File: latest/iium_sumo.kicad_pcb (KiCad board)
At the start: 2 copper layers, 56 parts, among them J1 I2C_VL53_1, J10 Cytron MD, J11 Cytron Start Module, J12 Conn_01x04, J13 Conn_01x04, J14 Conn_01x04, J15 EXTRA1, J16 Conn_01x02_Pin, J17 Conn_01x02_Pin, J18 UART1, J19 UART2, J2 I2C_VL53_2, J3 I2C_VL53_3, J4 I2C_VL53_4, J5 I2C_VL53_5, J6 IR_1, J7 IR_2, J8 IR_3, J9 IR_4, SW1 SW_SPST, SW2 SW_SPST, U1 TPS54360DDA, U4 Black Pill v2, U5 LM3940

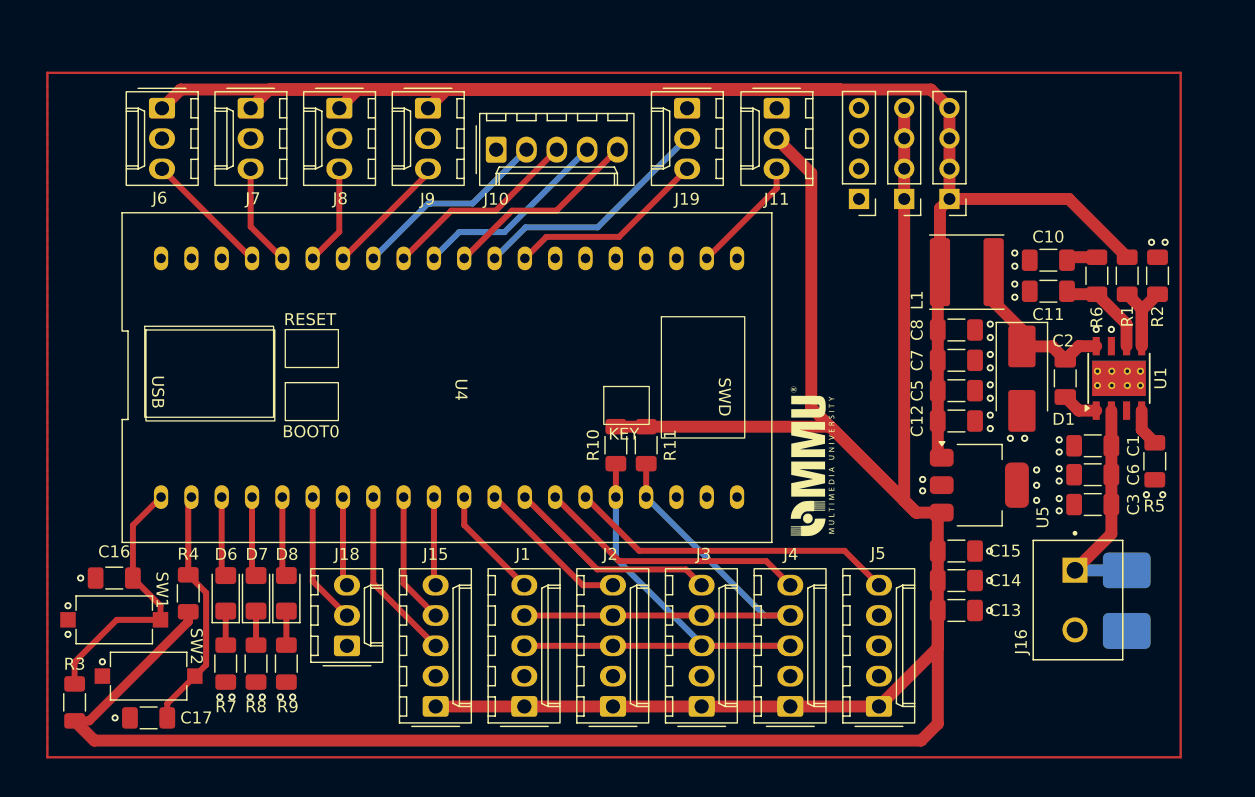
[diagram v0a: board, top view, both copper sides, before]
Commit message: drc cleared
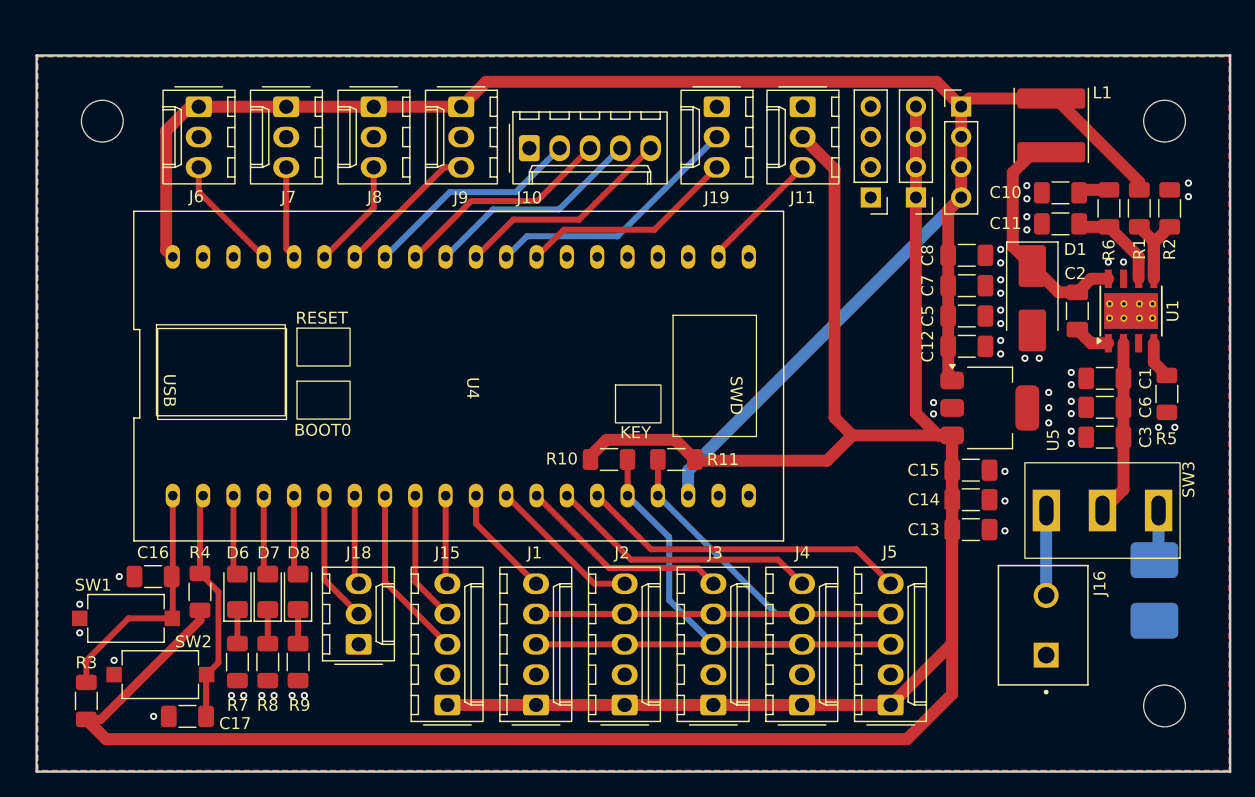
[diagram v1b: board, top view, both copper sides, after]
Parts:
- removed G***: LOGO, shooter_foot_library:mmu_logo
- added REF**: MountingHole_3.5mm, MountingHole:MountingHole_3.5mm, F.Cu at (105.5, 65.5)
- added REF**: MountingHole_3.5mm, MountingHole:MountingHole_3.5mm, F.Cu at (194.5, 65.5)
- added REF**: MountingHole_3.5mm, MountingHole:MountingHole_3.5mm, F.Cu at (194.5, 114.5)
- added SW3: SW_SPDT, custom:SPDT_MT-1-102-A001-M200-RS, F.Cu at (189.3, 98.1)
- moved L1 14.2 mm to (185.0, 65.9), turned to 90 degrees
- moved J13 7.81 mm to (177.5, 64.3), turned to 0 degrees
- moved C13 6.88 mm to (178.3, 99.7)
- moved C14 6.88 mm to (178.3, 97.2)
- moved C15 6.88 mm to (178.3, 94.7)
- moved D1 6.79 mm to (183.4, 80.3)
- moved U5 6.53 mm to (179.9, 89.5)
- moved C7 6.32 mm to (177.9, 79.3)
- moved C12 6.32 mm to (177.9, 84.4)
- moved C5 6.32 mm to (177.9, 81.8)
- moved C8 6.32 mm to (177.9, 76.7)
- moved R1 5.74 mm to (192.4, 72.8)
- moved R2 5.74 mm to (194.9, 72.8)
- moved R6 5.74 mm to (189.8, 72.8)
- moved C1 5.74 mm to (189.5, 87.1)
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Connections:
- C1 pad 1: +36V -> Net-(SW3-B)
- C3 pad 1: +36V -> Net-(SW3-B)
- C6 pad 1: +36V -> Net-(SW3-B)
- J16 pad 1: +36V -> GND
- J16 pad 2: GND -> +36V
- J17 pad 1: +36V -> GND
- J17 pad 2: GND -> +36V
- U1 pad 2: +36V -> Net-(SW3-B)
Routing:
- net +5V: track 241.8 -> 156.7 mm
- net Net-(SW3-B): track 0.00 -> 14.7 mm
- net +36V: track 19.0 -> 11.4 mm
- net /I2C_SDA: track 41.6 -> 49.0 mm
- net /I2C_SCL: track 47.9 -> 55.2 mm
- net +3V3: track 253.6 -> 260.7 mm
- net Net-(D1-K): track 14.4 -> 20.2 mm
- net /PB12: track 22.7 -> 20.9 mm
- net /LEFT_DIR: track 16.8 -> 18.6 mm
- net /IR4_D0: track 10.5 -> 12.0 mm
- net /RIGHT_PWM: track 16.9 -> 18.4 mm
- net /LEFT_PWM: track 17.0 -> 18.5 mm
- net /TX2: track 20.3 -> 21.8 mm
- net /RX2: track 16.7 -> 18.2 mm
- net /RIGHT_DIR: track 17.1 -> 18.4 mm
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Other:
- board outline added: 100 x 60 mm

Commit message: relayout button
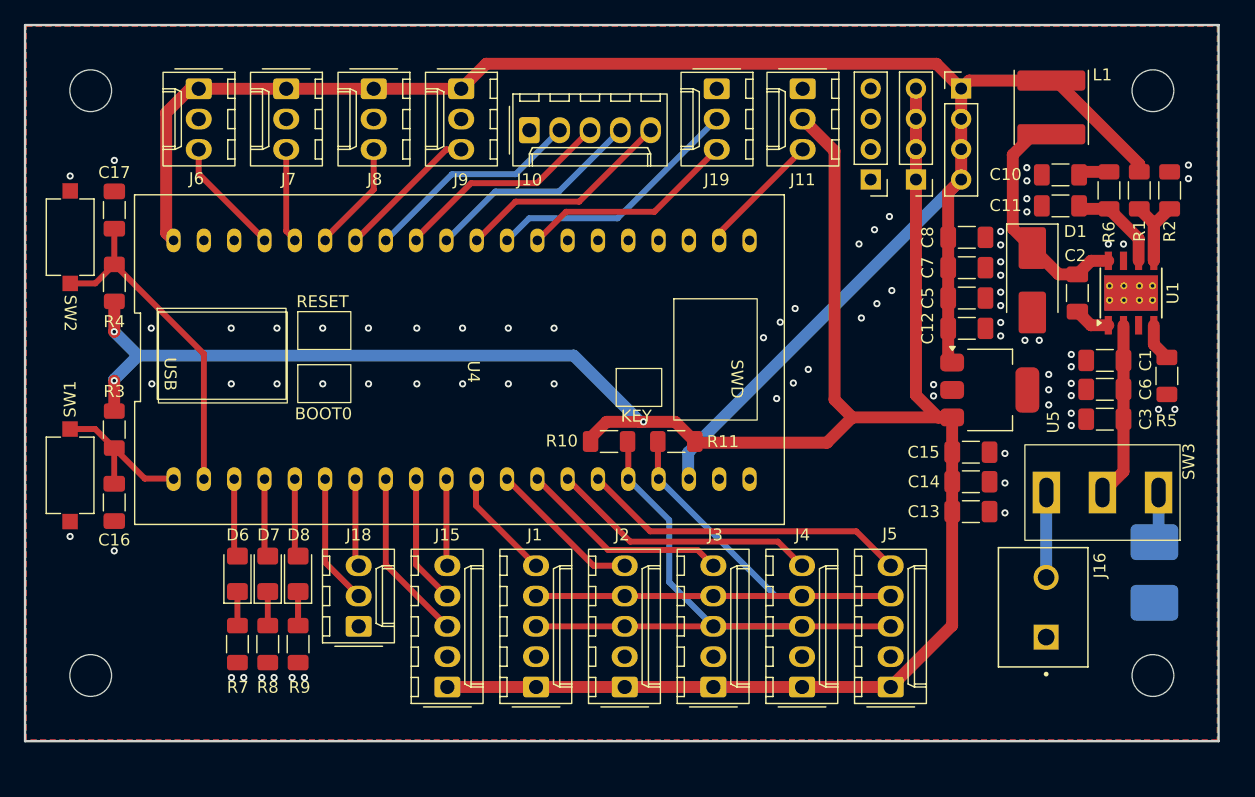
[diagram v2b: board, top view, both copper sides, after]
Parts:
- added REF**: MountingHole_3.5mm, MountingHole:MountingHole_3.5mm, F.Cu at (104.5, 112.0)
- moved C17 42.9 mm to (106.5, 73.0), turned to 90 degrees
- moved SW2 37.4 mm to (102.8, 75.2), turned to 90 degrees
- moved R4 26.9 mm to (106.5, 79.1)
- moved R3 22.9 mm to (106.5, 91.3), turned to -90 degrees
- moved SW1 12.9 mm to (102.8, 95.2), turned to -90 degrees
- moved C16 7.02 mm to (106.5, 97.4), turned to -90 degrees
- moved REF** 2.73 mm to (104.5, 63.0)
- moved REF** 2.73 mm to (193.5, 63.0)
- moved REF** 2.73 mm to (193.5, 112.0)
- moved C1 1.51 mm to (189.5, 85.5)
- moved C11 1.51 mm to (185.8, 72.6)
- moved C12 1.51 mm to (177.9, 82.9)
- moved C14 1.51 mm to (178.3, 95.7)
- moved C3 1.51 mm to (189.5, 90.5)
- moved C5 1.51 mm to (177.9, 80.3)
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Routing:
- net +3V3: track 260.7 -> 206.0 mm, vias 0 -> 3
- net /PB13: track 19.7 -> 28.4 mm
- net /PB12: track 20.9 -> 13.3 mm
- net GND: vias 45 -> 74
